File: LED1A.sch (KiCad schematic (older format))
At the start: 16 parts

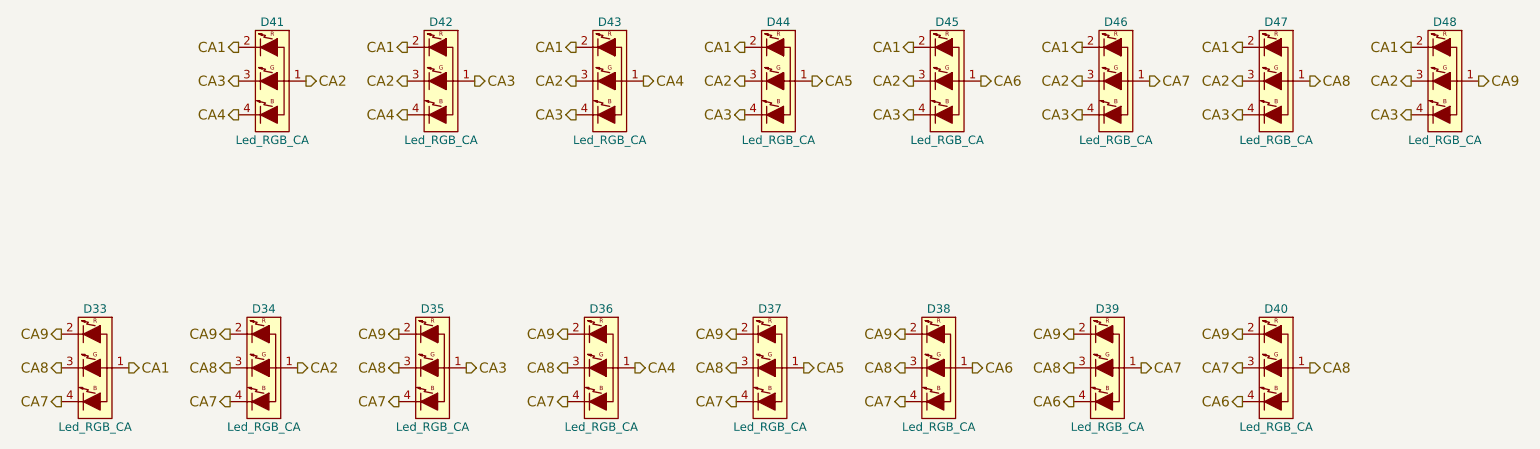
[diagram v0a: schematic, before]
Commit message: Did some visual cleanup.
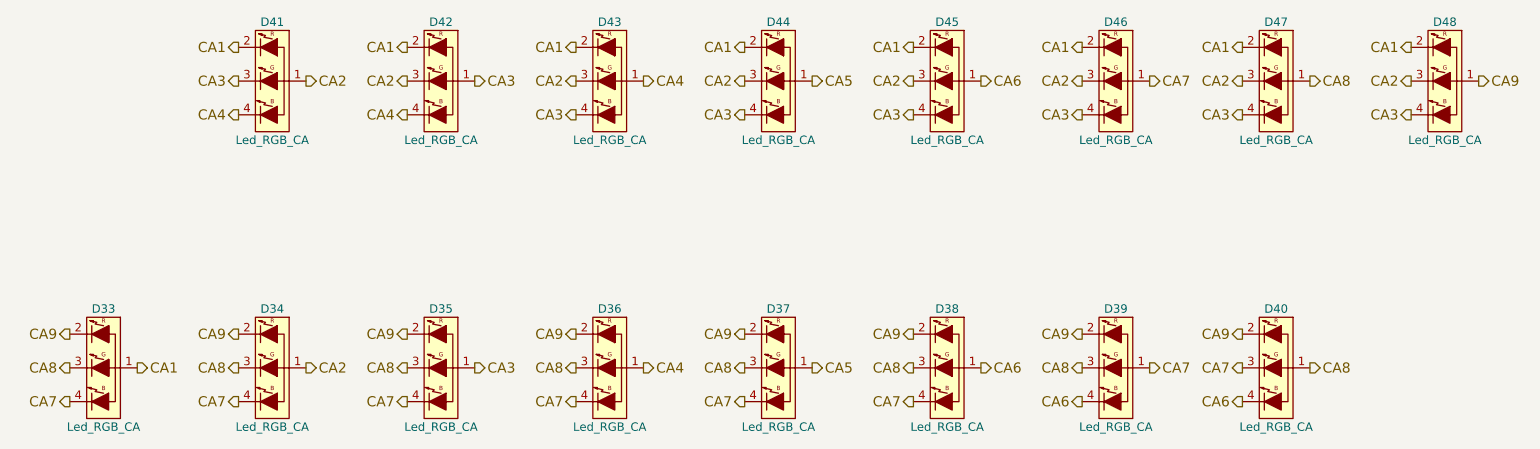
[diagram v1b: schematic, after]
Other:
- moved on the sheet: D33, D34, D35, D36, D37, D38, D39
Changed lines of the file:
@@
 $Descr A4 11693 8268
 encoding utf-8
-Sheet 4 6
+Sheet 5 6
 Title ""
 Date ""
@@
 Text HLabel 9750 1550 0    60   Output ~ 0
 CA1
-Text HLabel 2150 3450 2    60   Output ~ 0
-CA1
-Text HLabel 1750 3650 0    60   Output ~ 0
-CA7
-Text HLabel 1750 3450 0    60   Output ~ 0
-CA8
-Text HLabel 1750 3250 0    60   Output ~ 0
-CA9
-Text HLabel 2750 3650 0    60   Output ~ 0
-CA7
-Text HLabel 2750 3450 0    60   Output ~ 0
-CA8
-Text HLabel 2750 3250 0    60   Output ~ 0
-CA9
-Text HLabel 3150 3450 2    60   Output ~ 0
-CA2
-Text HLabel 3750 3650 0    60   Output ~ 0
-CA7
-Text HLabel 3750 3450 0    60   Output ~ 0
-CA8
-Text HLabel 3750 3250 0    60   Output ~ 0
-CA9
-Text HLabel 4150 3450 2    60   Output ~ 0
-CA3
-Text HLabel 4750 3650 0    60   Output ~ 0
-CA7
-Text HLabel 4750 3450 0    60   Output ~ 0
-CA8
-Text HLabel 4750 3250 0    60   Output ~ 0
-CA9
-Text HLabel 5150 3450 2    60   Output ~ 0
+Text HLabel 2200 3450 2    60   Output ~ 0
+CA1
+Text HLabel 1800 3650 0    60   Output ~ 0
+CA7
+Text HLabel 1800 3450 0    60   Output ~ 0
+CA8
+Text HLabel 1800 3250 0    60   Output ~ 0
+CA9
+Text HLabel 2800 3650 0    60   Output ~ 0
+CA7
+Text HLabel 2800 3450 0    60   Output ~ 0
+CA8
+Text HLabel 2800 3250 0    60   Output ~ 0
+CA9
+Text HLabel 3200 3450 2    60   Output ~ 0
+CA2
+Text HLabel 3800 3650 0    60   Output ~ 0
+CA7
+Text HLabel 3800 3450 0    60   Output ~ 0
+CA8
+Text HLabel 3800 3250 0    60   Output ~ 0
+CA9
+Text HLabel 4200 3450 2    60   Output ~ 0
+CA3
+Text HLabel 4800 3650 0    60   Output ~ 0
+CA7
+Text HLabel 4800 3450 0    60   Output ~ 0
+CA8
+Text HLabel 4800 3250 0    60   Output ~ 0
+CA9
+Text HLabel 5200 3450 2    60   Output ~ 0
 CA4
-Text HLabel 5750 3650 0    60   Output ~ 0
-CA7
-Text HLabel 5750 3450 0    60   Output ~ 0
-CA8
-Text HLabel 5750 3250 0    60   Output ~ 0
-CA9
-Text HLabel 6150 3450 2    60   Output ~ 0
+Text HLabel 5800 3650 0    60   Output ~ 0
+CA7
+Text HLabel 5800 3450 0    60   Output ~ 0
+CA8
+Text HLabel 5800 3250 0    60   Output ~ 0
+CA9
+Text HLabel 6200 3450 2    60   Output ~ 0
 CA5
-Text HLabel 6750 3650 0    60   Output ~ 0
-CA7
-Text HLabel 6750 3450 0    60   Output ~ 0
-CA8
-Text HLabel 6750 3250 0    60   Output ~ 0
-CA9
-Text HLabel 7150 3450 2    60   Output ~ 0
+Text HLabel 6800 3650 0    60   Output ~ 0
+CA7
+Text HLabel 6800 3450 0    60   Output ~ 0
+CA8
+Text HLabel 6800 3250 0    60   Output ~ 0
+CA9
+Text HLabel 7200 3450 2    60   Output ~ 0
 CA6
-Text HLabel 8150 3450 2    60   Output ~ 0
-CA7
-Text HLabel 7750 3450 0    60   Output ~ 0
-CA8
-Text HLabel 7750 3250 0    60   Output ~ 0
-CA9
-Text HLabel 7750 3650 0    60   Output ~ 0
+Text HLabel 8200 3450 2    60   Output ~ 0
+CA7
+Text HLabel 7800 3450 0    60   Output ~ 0
+CA8
+Text HLabel 7800 3250 0    60   Output ~ 0
+CA9
+Text HLabel 7800 3650 0    60   Output ~ 0
 CA6
 Text HLabel 8750 3250 0    60   Output ~ 0
@@
 L Led_RGB_CA D33
 U 1 1 56C9C1A0
-P 1950 3450
-F 0 "D33" H 1950 3800 50  0000 C CNN
-F 1 "Led_RGB_CA" H 1950 3100 50  0000 C CNN
-F 2 "mx2a:RGB" H 1905 3400 50  0001 C CNN
-F 3 "" H 1905 3400 50  0000 C CNN
-	1    1950 3450
+P 2000 3450
+F 0 "D33" H 2000 3800 50  0000 C CNN
+F 1 "Led_RGB_CA" H 2000 3100 50  0000 C CNN
+F 2 "mx2a:RGB" H 1955 3400 50  0001 C CNN
+F 3 "" H 1955 3400 50  0000 C CNN
+	1    2000 3450
 	1    0    0    -1
 $EndComp
@@
 L Led_RGB_CA D34
 U 1 1 56C9C3B3
-P 2950 3450
-F 0 "D34" H 2950 3800 50  0000 C CNN
-F 1 "Led_RGB_CA" H 2950 3100 50  0000 C CNN
-F 2 "mx2a:RGB" H 2905 3400 50  0001 C CNN
-F 3 "" H 2905 3400 50  0000 C CNN
-	1    2950 3450
+P 3000 3450
+F 0 "D34" H 3000 3800 50  0000 C CNN
+F 1 "Led_RGB_CA" H 3000 3100 50  0000 C CNN
+F 2 "mx2a:RGB" H 2955 3400 50  0001 C CNN
+F 3 "" H 2955 3400 50  0000 C CNN
+	1    3000 3450
 	1    0    0    -1
 $EndComp
@@
 L Led_RGB_CA D35
 U 1 1 56C9C4F1
-P 3950 3450
-F 0 "D35" H 3950 3800 50  0000 C CNN
-F 1 "Led_RGB_CA" H 3950 3100 50  0000 C CNN
-F 2 "mx2a:RGB" H 3905 3400 50  0001 C CNN
-F 3 "" H 3905 3400 50  0000 C CNN
-	1    3950 3450
+P 4000 3450
+F 0 "D35" H 4000 3800 50  0000 C CNN
+F 1 "Led_RGB_CA" H 4000 3100 50  0000 C CNN
+F 2 "mx2a:RGB" H 3955 3400 50  0001 C CNN
+F 3 "" H 3955 3400 50  0000 C CNN
+	1    4000 3450
 	1    0    0    -1
 $EndComp
@@
 L Led_RGB_CA D36
 U 1 1 56C9C542
-P 4950 3450
-F 0 "D36" H 4950 3800 50  0000 C CNN
-F 1 "Led_RGB_CA" H 4950 3100 50  0000 C CNN
-F 2 "mx2a:RGB" H 4905 3400 50  0001 C CNN
-F 3 "" H 4905 3400 50  0000 C CNN
-	1    4950 3450
+P 5000 3450
+F 0 "D36" H 5000 3800 50  0000 C CNN
+F 1 "Led_RGB_CA" H 5000 3100 50  0000 C CNN
+F 2 "mx2a:RGB" H 4955 3400 50  0001 C CNN
+F 3 "" H 4955 3400 50  0000 C CNN
+	1    5000 3450
 	1    0    0    -1
 $EndComp
@@
 L Led_RGB_CA D37
 U 1 1 56C9C7EA
-P 5950 3450
-F 0 "D37" H 5950 3800 50  0000 C CNN
-F 1 "Led_RGB_CA" H 5950 3100 50  0000 C CNN
-F 2 "mx2a:RGB" H 5905 3400 50  0001 C CNN
-F 3 "" H 5905 3400 50  0000 C CNN
-	1    5950 3450
+P 6000 3450
+F 0 "D37" H 6000 3800 50  0000 C CNN
+F 1 "Led_RGB_CA" H 6000 3100 50  0000 C CNN
+F 2 "mx2a:RGB" H 5955 3400 50  0001 C CNN
+F 3 "" H 5955 3400 50  0000 C CNN
+	1    6000 3450
 	1    0    0    -1
 $EndComp
@@
 L Led_RGB_CA D38
 U 1 1 56C9CA10
-P 6950 3450
-F 0 "D38" H 6950 3800 50  0000 C CNN
-F 1 "Led_RGB_CA" H 6950 3100 50  0000 C CNN
-F 2 "mx2a:RGB" H 6905 3400 50  0001 C CNN
-F 3 "" H 6905 3400 50  0000 C CNN
-	1    6950 3450
+P 7000 3450
+F 0 "D38" H 7000 3800 50  0000 C CNN
+F 1 "Led_RGB_CA" H 7000 3100 50  0000 C CNN
+F 2 "mx2a:RGB" H 6955 3400 50  0001 C CNN
+F 3 "" H 6955 3400 50  0000 C CNN
+	1    7000 3450
 	1    0    0    -1
 $EndComp
@@
 L Led_RGB_CA D39
 U 1 1 56C9CA6E
-P 7950 3450
-F 0 "D39" H 7950 3800 50  0000 C CNN
-F 1 "Led_RGB_CA" H 7950 3100 50  0000 C CNN
-F 2 "mx2a:RGB" H 7905 3400 50  0001 C CNN
-F 3 "" H 7905 3400 50  0000 C CNN
-	1    7950 3450
-	1    0    0    -1
-$EndComp
+P 8000 3450
+F 0 "D39" H 8000 3800 50  0000 C CNN
+F 1 "Led_RGB_CA" H 8000 3100 50  0000 C CNN
+F 2 "mx2a:RGB" H 7955 3400 50  0001 C CNN
+F 3 "" H 7955 3400 50  0000 C CNN
+	1    8000 3450
+	1    0    0    -1
+$EndComp

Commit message: Switched to a different USB Port and 100uF Cap
also added a USB-Debug Header and did some cleanup
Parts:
- D33, D34, D35, D36, D37, D38, D39, D40, D41, D42, D43, D44, D45, D46, D47, D48: footprint mx2a:RGB -> libs.pretty:RGB
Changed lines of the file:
@@
 U 1 1 56C92051
 P 3000 1750
+AR Path="/56C92051" Ref="D41"  Part="1"
+AR Path="/576E55C2/56C92051" Ref="D41"  Part="1"
 F 0 "D41" H 3000 2100 50  0000 C CNN
 F 1 "Led_RGB_CA" H 3000 1400 50  0000 C CNN
-F 2 "mx2a:RGB" H 2955 1700 50  0001 C CNN
+F 2 "libs.pretty:RGB" H 2955 1700 50  0001 C CNN
 F 3 "" H 2955 1700 50  0000 C CNN
 	1    3000 1750
@@
 U 1 1 56C9208F
 P 4000 1750
+AR Path="/56C9208F" Ref="D42"  Part="1"
+AR Path="/576E55C2/56C9208F" Ref="D42"  Part="1"
 F 0 "D42" H 4000 2100 50  0000 C CNN
 F 1 "Led_RGB_CA" H 4000 1400 50  0000 C CNN
-F 2 "mx2a:RGB" H 3955 1700 50  0001 C CNN
+F 2 "libs.pretty:RGB" H 3955 1700 50  0001 C CNN
 F 3 "" H 3955 1700 50  0000 C CNN
 	1    4000 1750
@@
 U 1 1 56C920ED
 P 5000 1750
+AR Path="/56C920ED" Ref="D43"  Part="1"
+AR Path="/576E55C2/56C920ED" Ref="D43"  Part="1"
 F 0 "D43" H 5000 2100 50  0000 C CNN
 F 1 "Led_RGB_CA" H 5000 1400 50  0000 C CNN
-F 2 "mx2a:RGB" H 4955 1700 50  0001 C CNN
+F 2 "libs.pretty:RGB" H 4955 1700 50  0001 C CNN
 F 3 "" H 4955 1700 50  0000 C CNN
 	1    5000 1750
@@
 U 1 1 56C921B4
 P 6000 1750
+AR Path="/56C921B4" Ref="D44"  Part="1"
+AR Path="/576E55C2/56C921B4" Ref="D44"  Part="1"
 F 0 "D44" H 6000 2100 50  0000 C CNN
 F 1 "Led_RGB_CA" H 6000 1400 50  0000 C CNN
-F 2 "mx2a:RGB" H 5955 1700 50  0001 C CNN
+F 2 "libs.pretty:RGB" H 5955 1700 50  0001 C CNN
 F 3 "" H 5955 1700 50  0000 C CNN
 	1    6000 1750
@@
 U 1 1 56C921EC
 P 7000 1750
+AR Path="/56C921EC" Ref="D45"  Part="1"
+AR Path="/576E55C2/56C921EC" Ref="D45"  Part="1"
 F 0 "D45" H 7000 2100 50  0000 C CNN
 F 1 "Led_RGB_CA" H 7000 1400 50  0000 C CNN
-F 2 "mx2a:RGB" H 6955 1700 50  0001 C CNN
+F 2 "libs.pretty:RGB" H 6955 1700 50  0001 C CNN
 F 3 "" H 6955 1700 50  0000 C CNN
 	1    7000 1750
@@
 U 1 1 56C923D6
 P 8000 1750
+AR Path="/56C923D6" Ref="D46"  Part="1"
+AR Path="/576E55C2/56C923D6" Ref="D46"  Part="1"
 F 0 "D46" H 8000 2100 50  0000 C CNN
 F 1 "Led_RGB_CA" H 8000 1400 50  0000 C CNN
-F 2 "mx2a:RGB" H 7955 1700 50  0001 C CNN
+F 2 "libs.pretty:RGB" H 7955 1700 50  0001 C CNN
 F 3 "" H 7955 1700 50  0000 C CNN
 	1    8000 1750
@@
 U 1 1 56C92438
 P 8950 1750
+AR Path="/56C92438" Ref="D47"  Part="1"
+AR Path="/576E55C2/56C92438" Ref="D47"  Part="1"
 F 0 "D47" H 8950 2100 50  0000 C CNN
 F 1 "Led_RGB_CA" H 8950 1400 50  0000 C CNN
-F 2 "mx2a:RGB" H 8905 1700 50  0001 C CNN
+F 2 "libs.pretty:RGB" H 8905 1700 50  0001 C CNN
 F 3 "" H 8905 1700 50  0000 C CNN
 	1    8950 1750
@@
 U 1 1 56C9247D
 P 9950 1750
+AR Path="/56C9247D" Ref="D48"  Part="1"
+AR Path="/576E55C2/56C9247D" Ref="D48"  Part="1"
 F 0 "D48" H 9950 2100 50  0000 C CNN
 F 1 "Led_RGB_CA" H 9950 1400 50  0000 C CNN
-F 2 "mx2a:RGB" H 9905 1700 50  0001 C CNN
+F 2 "libs.pretty:RGB" H 9905 1700 50  0001 C CNN
 F 3 "" H 9905 1700 50  0000 C CNN
 	1    9950 1750
@@
 U 1 1 56C9C1A0
 P 2000 3450
+AR Path="/56C9C1A0" Ref="D33"  Part="1"
+AR Path="/576E55C2/56C9C1A0" Ref="D33"  Part="1"
 F 0 "D33" H 2000 3800 50  0000 C CNN
 F 1 "Led_RGB_CA" H 2000 3100 50  0000 C CNN
-F 2 "mx2a:RGB" H 1955 3400 50  0001 C CNN
+F 2 "libs.pretty:RGB" H 1955 3400 50  0001 C CNN
 F 3 "" H 1955 3400 50  0000 C CNN
 	1    2000 3450
@@
 U 1 1 56C9C3B3
 P 3000 3450
+AR Path="/56C9C3B3" Ref="D34"  Part="1"
+AR Path="/576E55C2/56C9C3B3" Ref="D34"  Part="1"
 F 0 "D34" H 3000 3800 50  0000 C CNN
 F 1 "Led_RGB_CA" H 3000 3100 50  0000 C CNN
-F 2 "mx2a:RGB" H 2955 3400 50  0001 C CNN
+F 2 "libs.pretty:RGB" H 2955 3400 50  0001 C CNN
 F 3 "" H 2955 3400 50  0000 C CNN
 	1    3000 3450
@@
 U 1 1 56C9C4F1
 P 4000 3450
+AR Path="/56C9C4F1" Ref="D35"  Part="1"
+AR Path="/576E55C2/56C9C4F1" Ref="D35"  Part="1"
 F 0 "D35" H 4000 3800 50  0000 C CNN
 F 1 "Led_RGB_CA" H 4000 3100 50  0000 C CNN
-F 2 "mx2a:RGB" H 3955 3400 50  0001 C CNN
+F 2 "libs.pretty:RGB" H 3955 3400 50  0001 C CNN
 F 3 "" H 3955 3400 50  0000 C CNN
 	1    4000 3450
@@
 U 1 1 56C9C542
 P 5000 3450
+AR Path="/56C9C542" Ref="D36"  Part="1"
+AR Path="/576E55C2/56C9C542" Ref="D36"  Part="1"
 F 0 "D36" H 5000 3800 50  0000 C CNN
 F 1 "Led_RGB_CA" H 5000 3100 50  0000 C CNN
-F 2 "mx2a:RGB" H 4955 3400 50  0001 C CNN
+F 2 "libs.pretty:RGB" H 4955 3400 50  0001 C CNN
 F 3 "" H 4955 3400 50  0000 C CNN
 	1    5000 3450
@@
 U 1 1 56C9C7EA
 P 6000 3450
+AR Path="/56C9C7EA" Ref="D37"  Part="1"
+AR Path="/576E55C2/56C9C7EA" Ref="D37"  Part="1"
 F 0 "D37" H 6000 3800 50  0000 C CNN
 F 1 "Led_RGB_CA" H 6000 3100 50  0000 C CNN
-F 2 "mx2a:RGB" H 5955 3400 50  0001 C CNN
+F 2 "libs.pretty:RGB" H 5955 3400 50  0001 C CNN
 F 3 "" H 5955 3400 50  0000 C CNN
 	1    6000 3450
@@
 U 1 1 56C9CA10
 P 7000 3450
+AR Path="/56C9CA10" Ref="D38"  Part="1"
+AR Path="/576E55C2/56C9CA10" Ref="D38"  Part="1"
 F 0 "D38" H 7000 3800 50  0000 C CNN
 F 1 "Led_RGB_CA" H 7000 3100 50  0000 C CNN
-F 2 "mx2a:RGB" H 6955 3400 50  0001 C CNN
+F 2 "libs.pretty:RGB" H 6955 3400 50  0001 C CNN
 F 3 "" H 6955 3400 50  0000 C CNN
 	1    7000 3450
@@
 U 1 1 56C9CA6E
 P 8000 3450
+AR Path="/56C9CA6E" Ref="D39"  Part="1"
+AR Path="/576E55C2/56C9CA6E" Ref="D39"  Part="1"
 F 0 "D39" H 8000 3800 50  0000 C CNN
 F 1 "Led_RGB_CA" H 8000 3100 50  0000 C CNN
-F 2 "mx2a:RGB" H 7955 3400 50  0001 C CNN
+F 2 "libs.pretty:RGB" H 7955 3400 50  0001 C CNN
 F 3 "" H 7955 3400 50  0000 C CNN
 	1    8000 3450
@@
 U 1 1 56C9CC74
 P 8950 3450
+AR Path="/56C9CC74" Ref="D40"  Part="1"
+AR Path="/576E55C2/56C9CC74" Ref="D40"  Part="1"
 F 0 "D40" H 8950 3800 50  0000 C CNN
 F 1 "Led_RGB_CA" H 8950 3100 50  0000 C CNN
-F 2 "mx2a:RGB" H 8905 3400 50  0001 C CNN
+F 2 "libs.pretty:RGB" H 8905 3400 50  0001 C CNN
 F 3 "" H 8905 3400 50  0000 C CNN
 	1    8950 3450
